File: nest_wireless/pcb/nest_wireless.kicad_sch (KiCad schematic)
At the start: 70 parts, among them J3 Conn_01x04, J4 FFC2B35-12-G_REVA2, SW1 SW_PUSH, SW10 SW_PUSH, SW11 SW_PUSH, SW12 SW_PUSH, SW13 SW_PUSH, SW14 SW_PUSH, SW15 SW_PUSH, SW16 SW_PUSH, SW17 SW_PUSH, SW18 SW_PUSH, SW19 SW_PUSH, SW2 SW_PUSH, SW20 SW_PUSH, SW21 SW_PUSH, SW22 SW_PUSH, SW23 SW_PUSH, SW24 SW_PUSH, SW25 Rotary_Encoder_Switch-Device, SW26 SW_PUSH, SW27 SW_PUSH, SW28 SW_PUSH, SW3 SW_PUSH, SW4 SW_PUSH, SW5 SW_PUSH, SW6 SW_PUSH, SW7 SW_PUSH, SW8 SW_PUSH, SW9 SW_PUSH, U2 kb2040

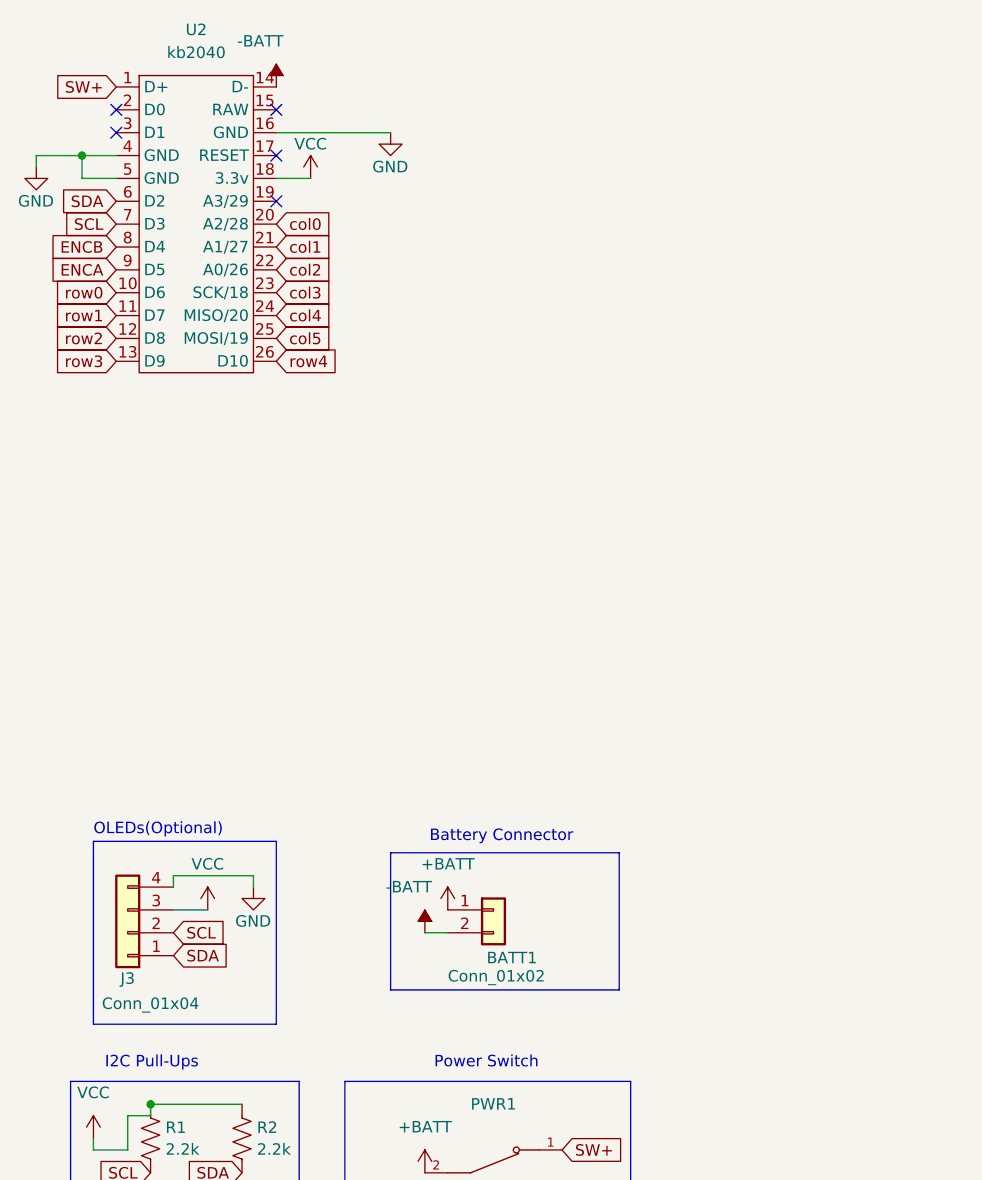
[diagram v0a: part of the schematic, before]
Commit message: Nest wireless kicad project cleanup
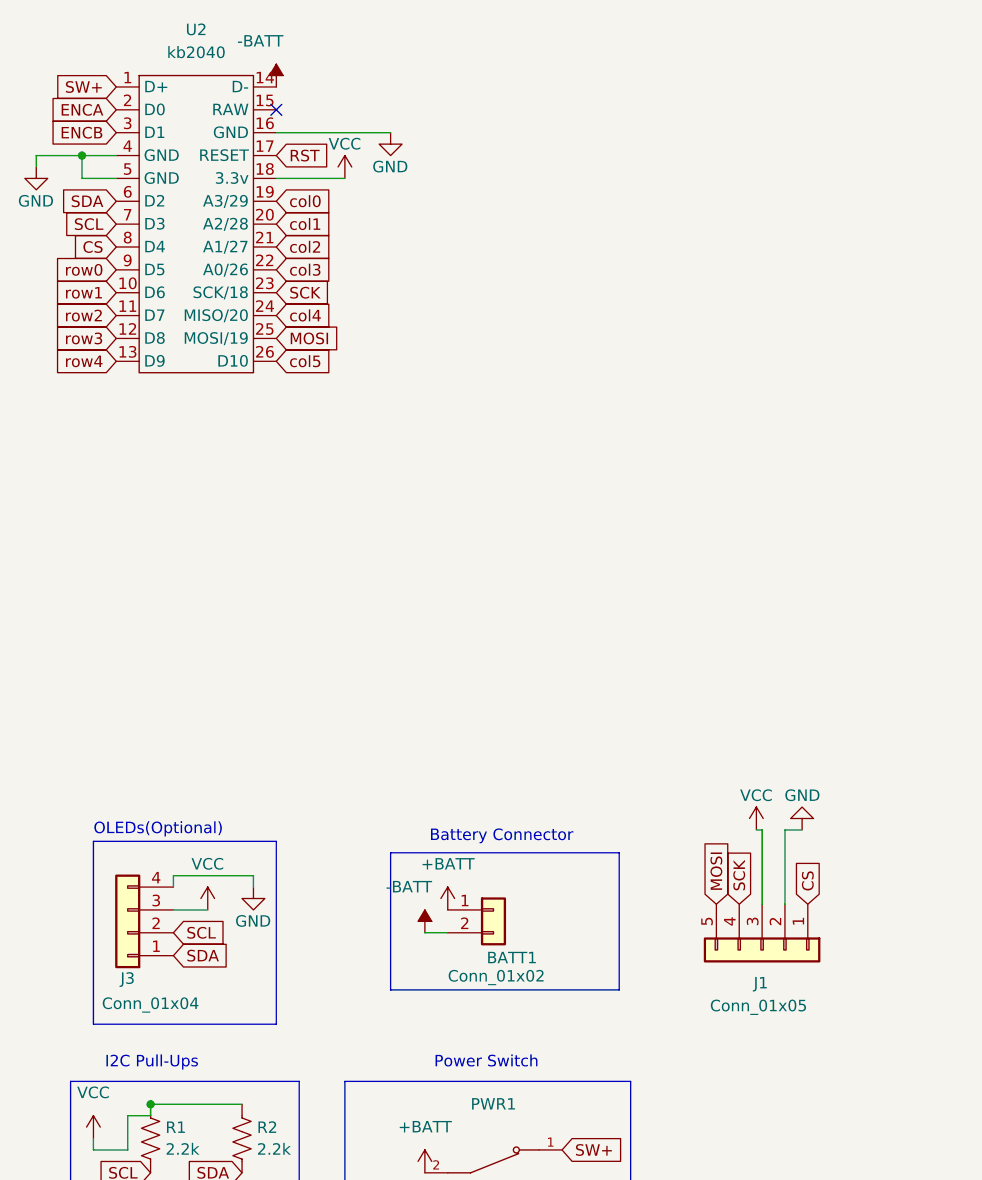
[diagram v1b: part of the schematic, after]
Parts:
- added J1: Conn_01x05, symbol Connector_Generic:Conn_01x05
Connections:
- net ENCA: now also U2.2 (D0); no longer U2.9 (D5)
- net ENCB: now also U2.3 (D1); no longer U2.8 (D4)
- net GND: now also J1.2 (Pin_2)
- net VCC: now also J1.3 (Pin_3)
- net col0: now also U2.19 (A3/29); no longer U2.20 (A2/28)
- net col1: now also U2.20 (A2/28); no longer U2.21 (A1/27)
- net col2: now also U2.21 (A1/27); no longer U2.22 (A0/26)
- net col3: now also U2.22 (A0/26); no longer U2.23 (SCK/18)
- net col5: now also U2.26 (D10); no longer U2.25 (MOSI/19)
- net row0: now also U2.9 (D5); no longer U2.10 (D6)
- net row1: now also U2.10 (D6); no longer U2.11 (D7)
- net row2: now also U2.11 (D7); no longer U2.12 (D8)
- net row3: now also U2.12 (D8); no longer U2.13 (D9)
- net row4: now also U2.13 (D9); no longer U2.26 (D10)
- net RST: now reaches U2.17 (RESET)
- new net CS: J1.1 (Pin_1), U2.8 (D4)
- new net MOSI: J1.5 (Pin_5), U2.25 (MOSI/19)
- new net SCK: J1.4 (Pin_4), U2.23 (SCK/18)
- no-connect marks 6 -> 2
